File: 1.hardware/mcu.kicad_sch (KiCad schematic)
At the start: 29 parts, among them J1 Debug, J2 usb_pwr, J3 vat_pwr, J4 ext_pwr, SW1 reset_btn, U1 STM32H743BITx, X1 SMD3225-4

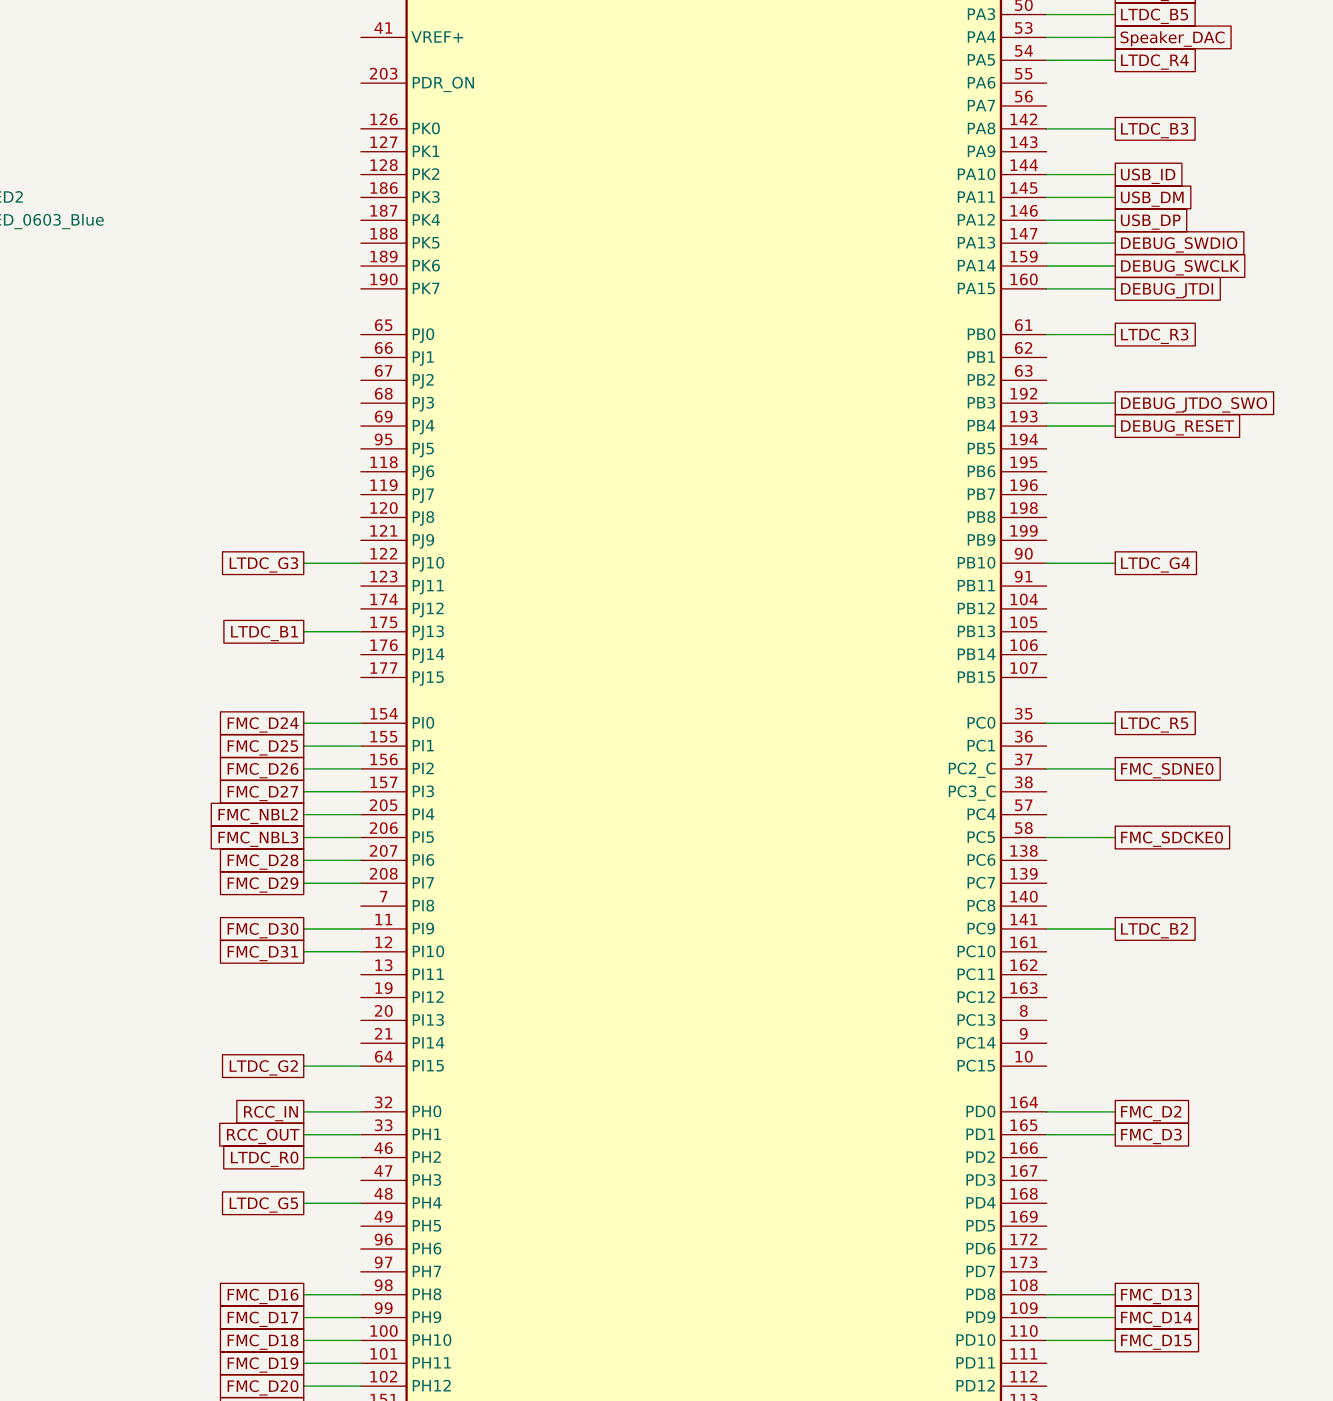
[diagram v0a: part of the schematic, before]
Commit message: 중간 저장2
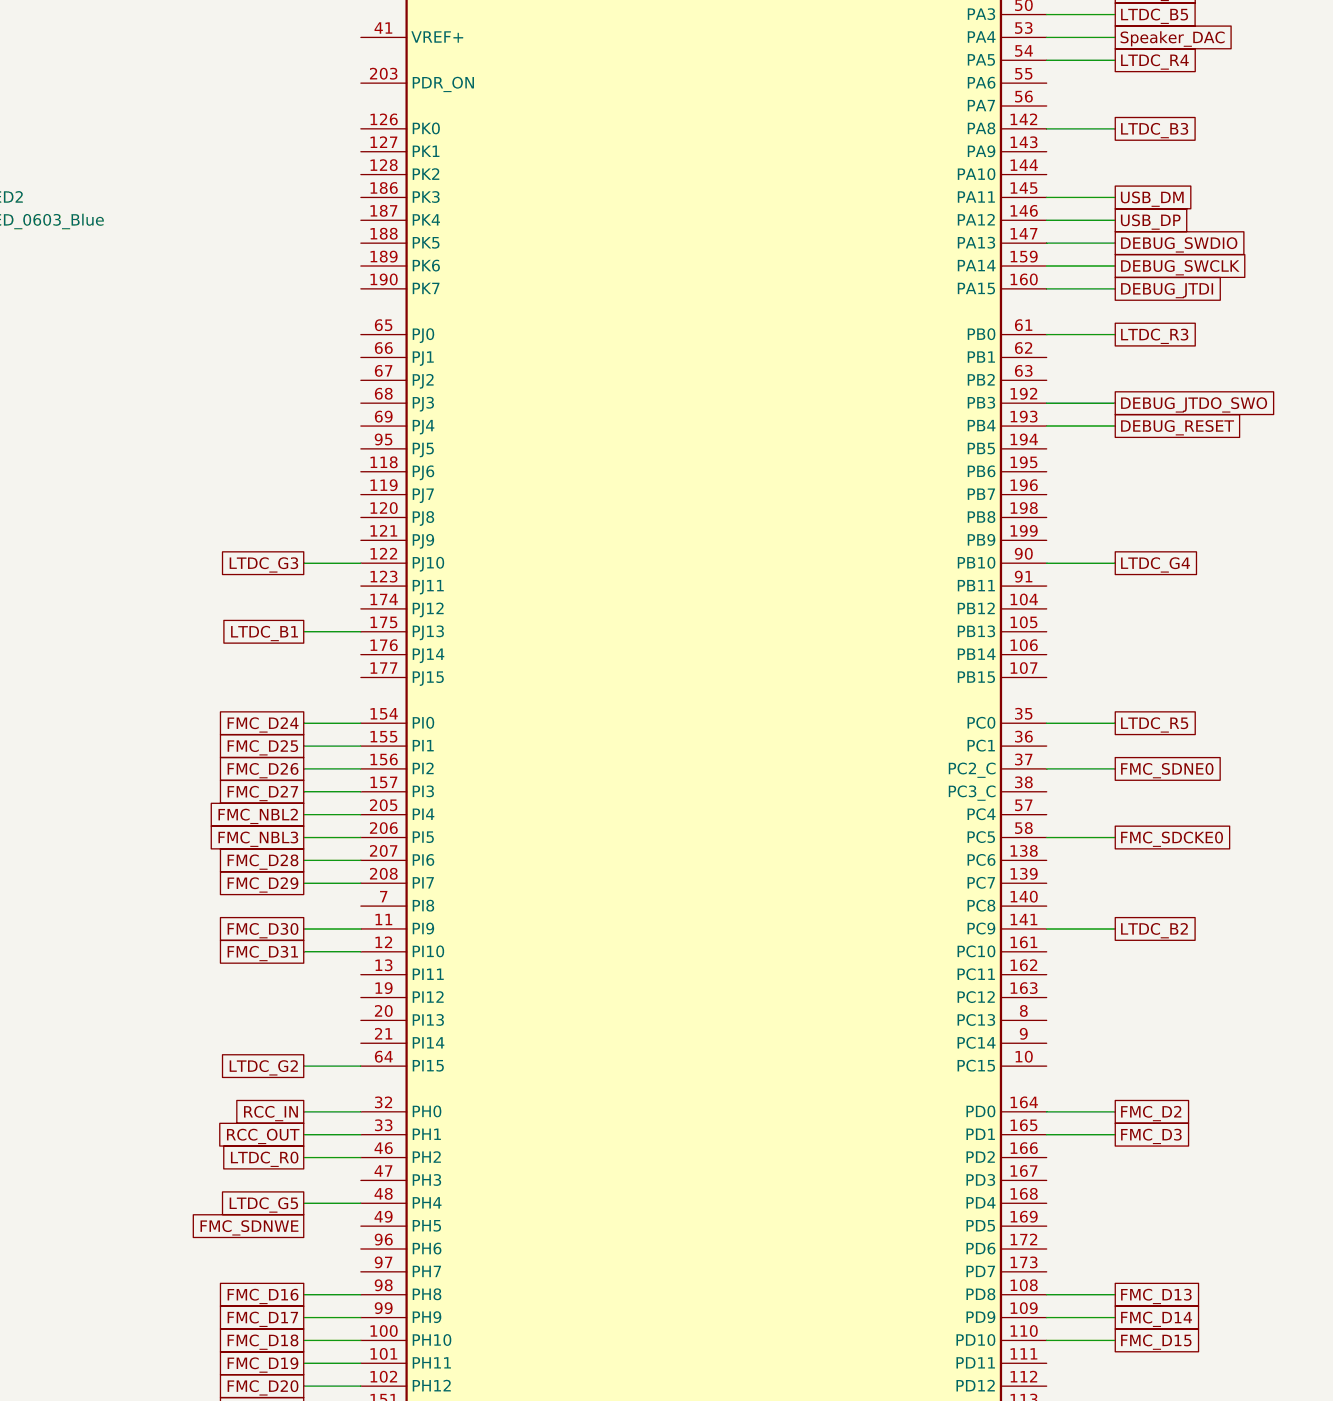
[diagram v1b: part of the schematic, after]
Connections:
- net USB_ID: no longer names the net of U1.144 (PA10)
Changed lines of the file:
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@@
-	(wire
-		(pts
-			(xy 321.31 106.68) (xy 328.93 106.68)
-		)
-		(stroke
-			(width 0)
-			(type default)
-		)
-	)
 	(wire
 		(pts
@@
 		)
 	)
+	(global_label "FMC_SDNWE"
+		(shape passive)
+		(at 238.76 223.52 180)
+		(fields_autoplaced yes)
+		(effects
+			(font
+				(size 1.27 1.27)
+			)
+			(justify right)
+		)
+		(property "Intersheetrefs" "${INTERSHEET_REFS}"
+			(at 225.6981 223.52 0)
+			(effects
+				(font
+					(size 1.27 1.27)
+				)
+				(justify right)
+				(hide yes)
+			)
+		)
+	)
 	(global_label "FMC_D17"
 		(shape passive)
@@
 			(effects
 				(font
-					(size 1.27 1.27)
-				)
-				(justify left)
-				(hide yes)
-			)
-		)
-	)
-	(global_label "USB_ID"
-		(shape passive)
-		(at 328.93 106.68 0)
-		(fields_autoplaced yes)
-		(effects
-			(font
-				(size 1.27 1.27)
-			)
-			(justify left)
-		)
-		(property "Intersheetrefs" "${INTERSHEET_REFS}"
-			(at 337.4563 106.68 0)
-			(effects
-				(font
